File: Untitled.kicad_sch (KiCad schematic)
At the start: 20 parts, among them J1 Battery Connector, J2 Top Screw Terminal, J3 Bottom Screw Terminal, Q1 Q_NMOS_DGS, Q2 Q_NMOS_DGS, Q3 Q_NMOS_DGS, U1 XIAO-ESP32-S3-SMD, U3 LSM6DSO32, U4 MS5611-01BA

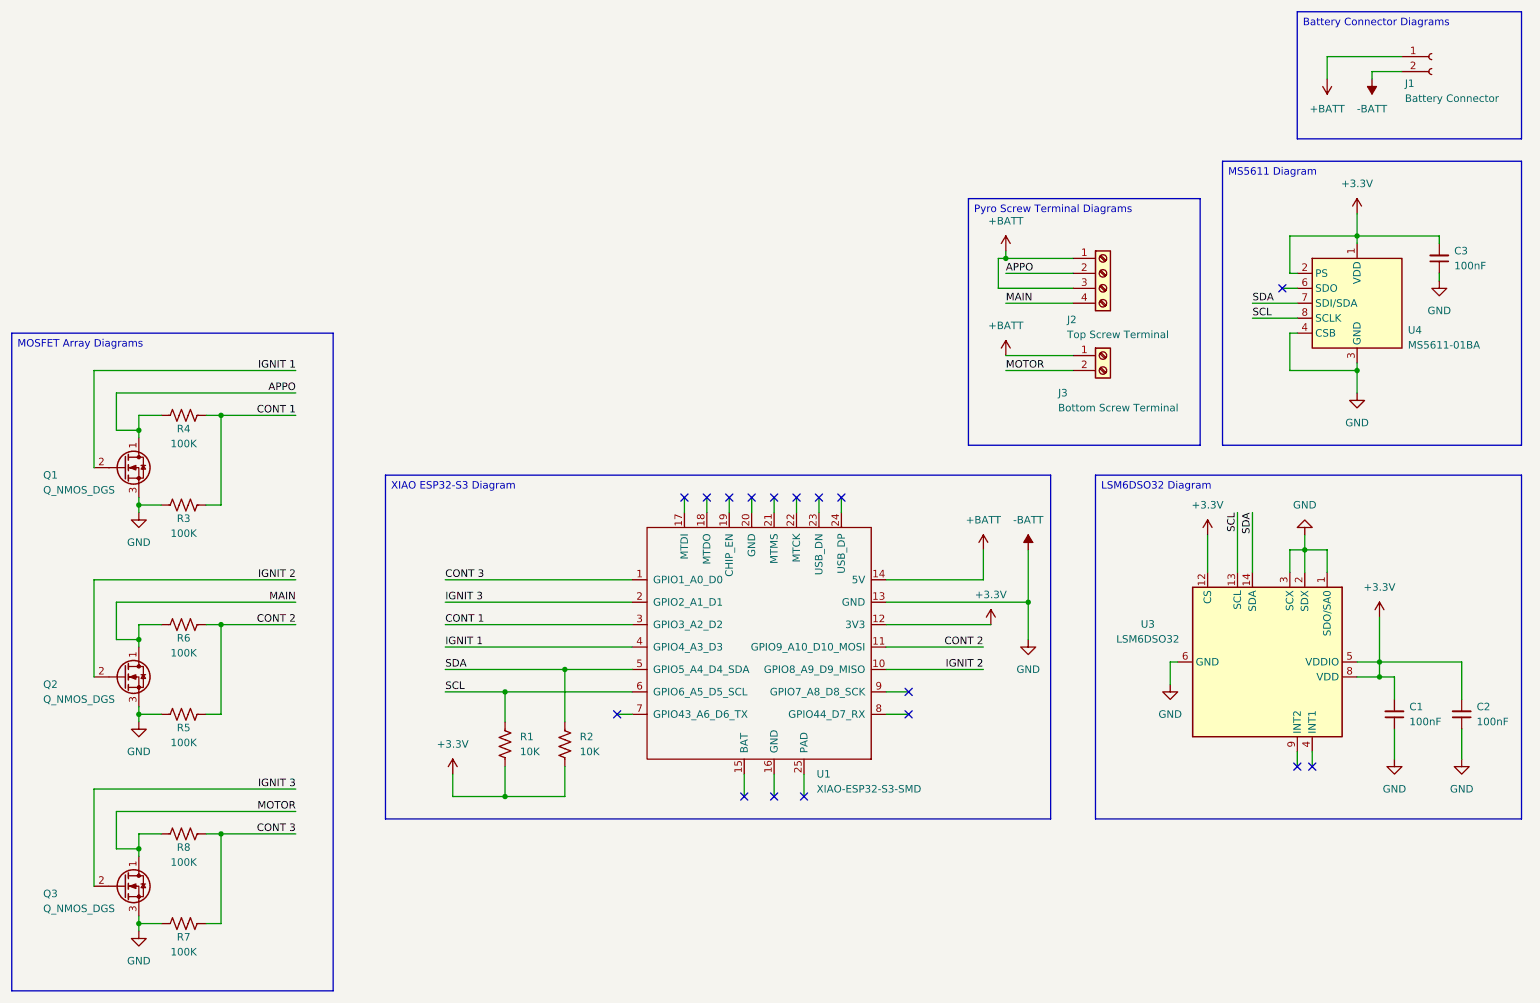
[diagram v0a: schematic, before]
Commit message: Small Changes
Did some small changes to silkscreen formatting.
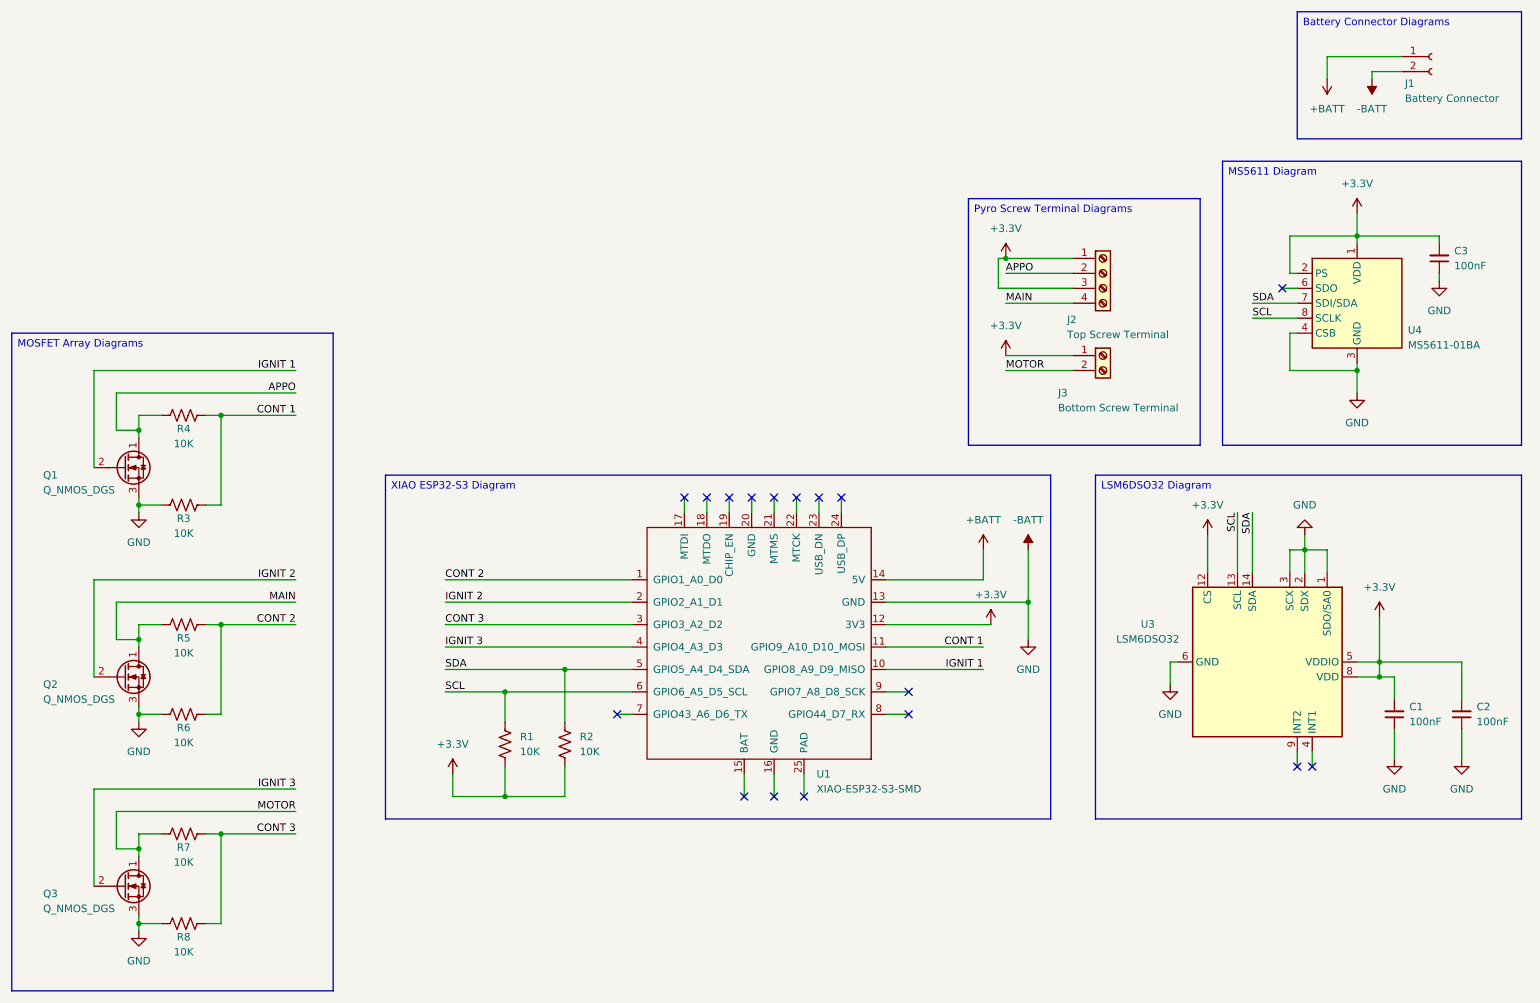
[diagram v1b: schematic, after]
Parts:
- R3, R4: value 100K -> 10K
- R5: renamed from R6; value 100K -> 10K
- R6: renamed from R5; value 100K -> 10K
- R7: renamed from R8; value 100K -> 10K
- R8: renamed from R7; value 100K -> 10K
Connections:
- net +3.3V: now also J2.1 (Pin_1), J2.3 (Pin_3), J3.1 (Pin_1)
- net +BATT: no longer J2.1 (Pin_1), J2.3 (Pin_3), J3.1 (Pin_1)
- net CONT 1: now also U1.11 (GPIO9_A10_D10_MOSI); no longer U1.3 (GPIO3_A2_D2)
- net CONT 2: now also U1.1 (GPIO1_A0_D0); no longer U1.11 (GPIO9_A10_D10_MOSI)
- net CONT 3: now also U1.3 (GPIO3_A2_D2); no longer U1.1 (GPIO1_A0_D0)
- net IGNIT 1: now also U1.10 (GPIO8_A9_D9_MISO); no longer U1.4 (GPIO4_A3_D3)
- net IGNIT 2: now also U1.2 (GPIO2_A1_D1); no longer U1.10 (GPIO8_A9_D9_MISO)
- net IGNIT 3: now also U1.4 (GPIO4_A3_D3); no longer U1.2 (GPIO2_A1_D1)

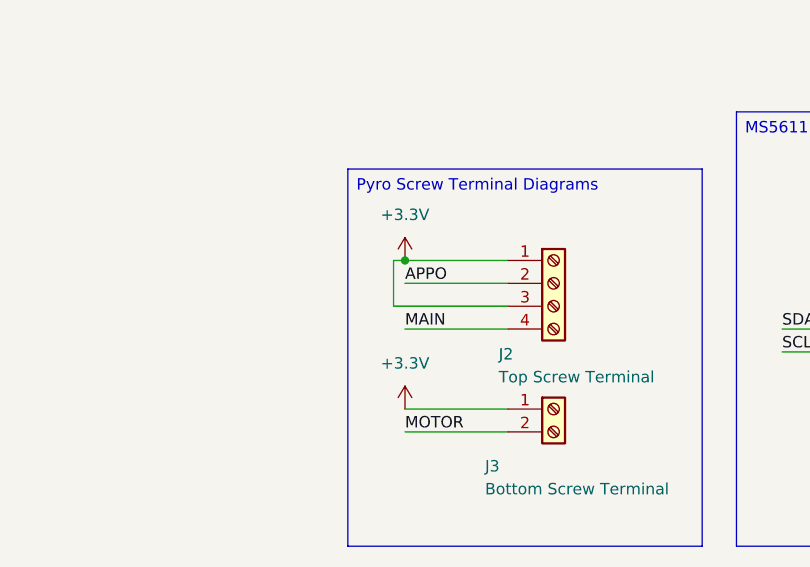
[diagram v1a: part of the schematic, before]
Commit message: Added cutouts, spaced rod holes
Added cutouts to the side of the PCB for wires to pass through on both sides of the ESP32. Changed distance between screw holes to accurately reflect the spacing used for threaded rods on previous avionics designs.
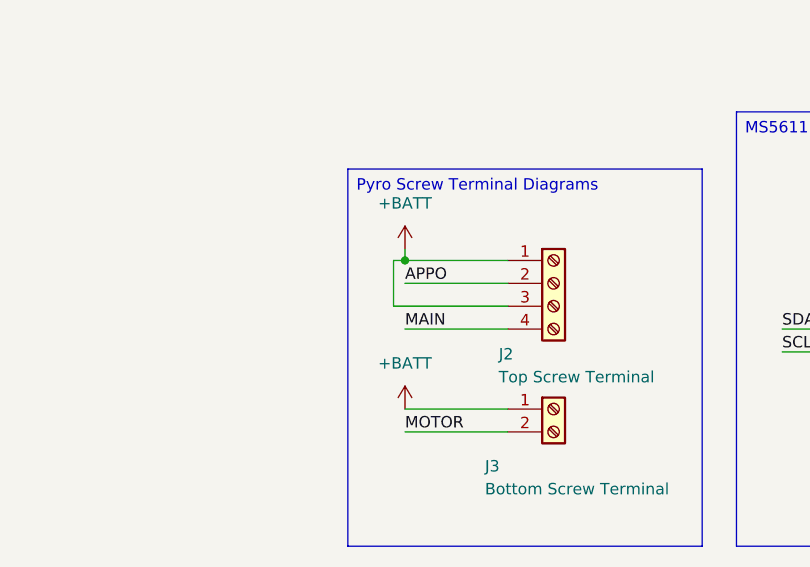
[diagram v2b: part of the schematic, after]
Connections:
- net +3.3V: no longer J2.1 (Pin_1), J2.3 (Pin_3), J3.1 (Pin_1)
- net +BATT: now also J2.1 (Pin_1), J2.3 (Pin_3), J3.1 (Pin_1)

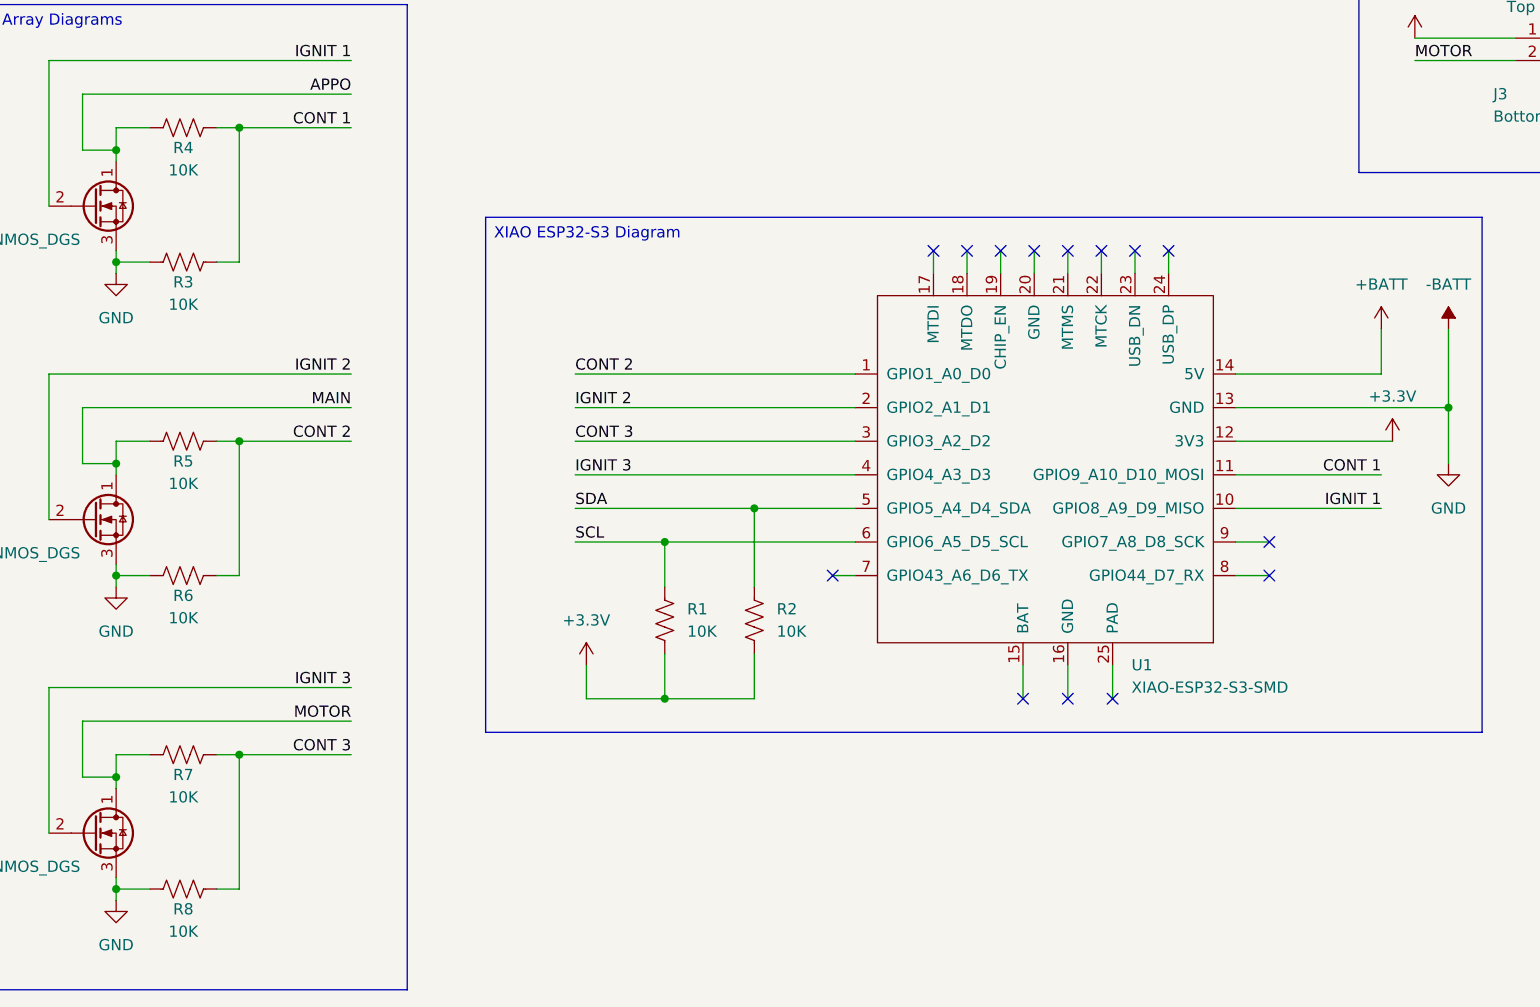
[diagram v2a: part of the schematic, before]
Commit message: Initial Routing
Completed initial manual routing of PCB traces. All nets are fully connected.
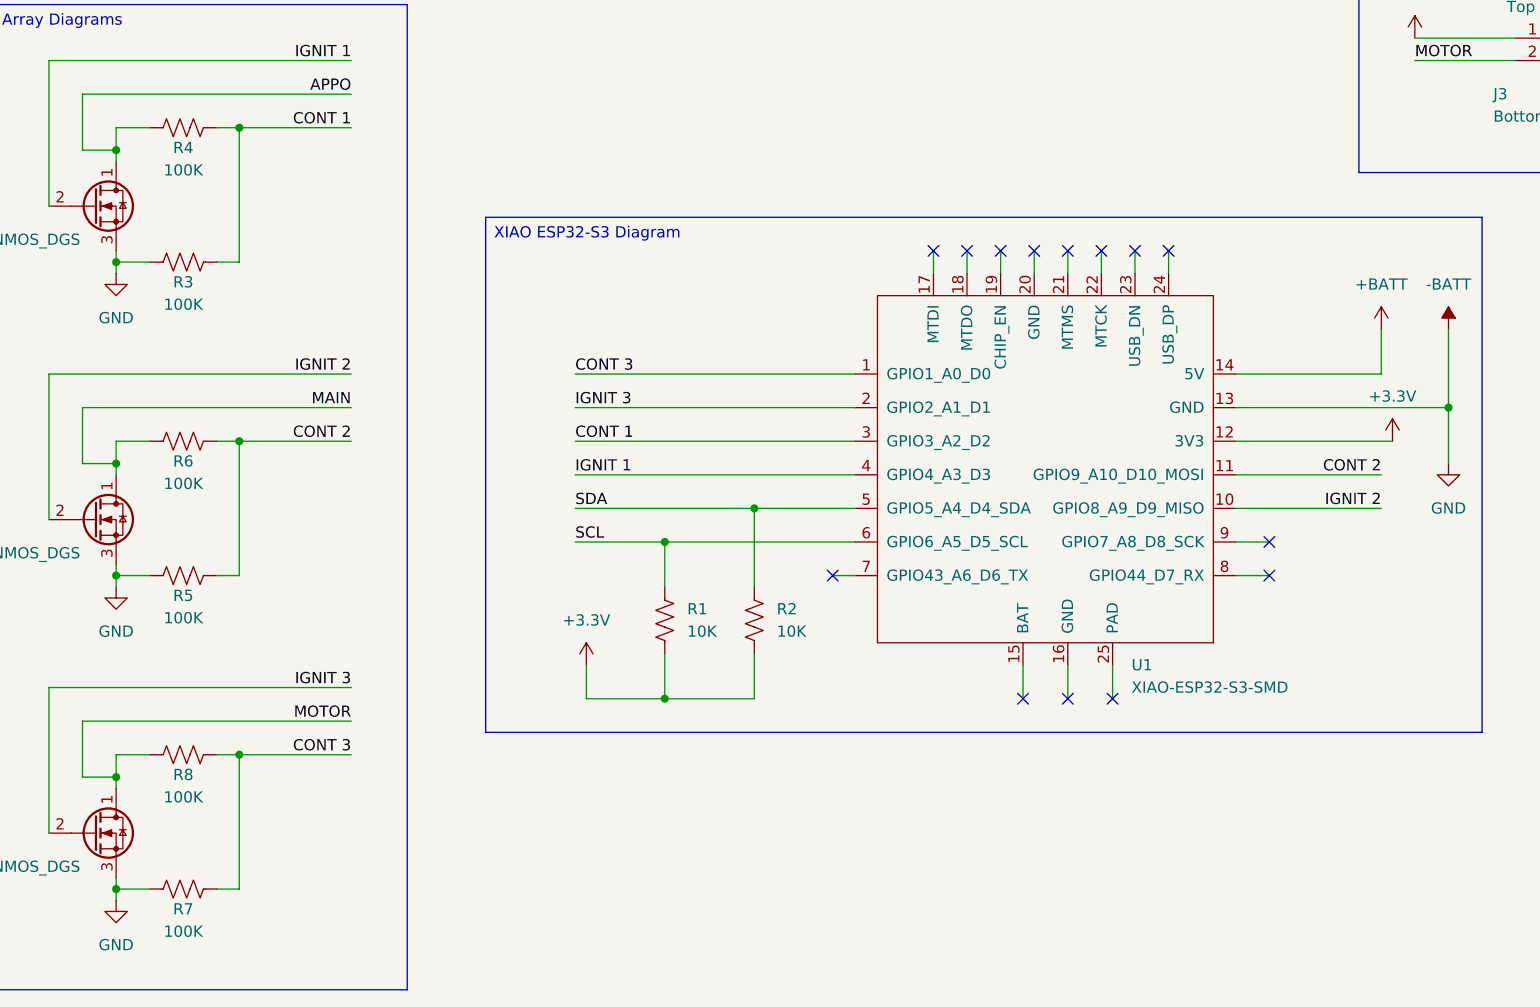
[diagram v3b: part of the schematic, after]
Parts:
- R3, R4: value 10K -> 100K
- R5: renamed from R6; value 10K -> 100K
- R6: renamed from R5; value 10K -> 100K
- R7: renamed from R8; value 10K -> 100K
- R8: renamed from R7; value 10K -> 100K
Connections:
- net CONT 1: now also U1.3 (GPIO3_A2_D2); no longer U1.11 (GPIO9_A10_D10_MOSI)
- net CONT 2: now also U1.11 (GPIO9_A10_D10_MOSI); no longer U1.1 (GPIO1_A0_D0)
- net CONT 3: now also U1.1 (GPIO1_A0_D0); no longer U1.3 (GPIO3_A2_D2)
- net IGNIT 1: now also U1.4 (GPIO4_A3_D3); no longer U1.10 (GPIO8_A9_D9_MISO)
- net IGNIT 2: now also U1.10 (GPIO8_A9_D9_MISO); no longer U1.2 (GPIO2_A1_D1)
- net IGNIT 3: now also U1.2 (GPIO2_A1_D1); no longer U1.4 (GPIO4_A3_D3)
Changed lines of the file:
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@@
 		)
 	)
-	(label "IGNIT 1"
+	(label "IGNIT 2"
 		(at 187.96 137.16 180)
 		(effects
@@
 		)
 	)
-	(label "IGNIT 2"
+	(label "IGNIT 3"
 		(at 96.52 125.73 0)
 		(effects
@@
 		)
 	)
-	(label "CONT 1"
+	(label "CONT 2"
 		(at 187.96 133.35 180)
 		(effects
@@
 		)
 	)
-	(label "IGNIT 3"
+	(label "IGNIT 1"
 		(at 96.52 133.35 0)
 		(effects
@@
 		)
 	)
-	(label "CONT 3"
+	(label "CONT 1"
 		(at 96.52 129.54 0)
 		(effects
@@
 		)
 	)
-	(label "CONT 2"
+	(label "CONT 3"
 		(at 96.52 121.92 0)
 		(effects
@@
 			)
 		)
-		(property "Value" "10K"
+		(property "Value" "100K"
 			(at 52.07 98.806 90)
 			(effects
@@
 		(on_board yes)
 		(dnp no)
-		(property "Reference" "R6"
+		(property "Reference" "R5"
 			(at 52.07 147.066 90)
 			(effects
@@
 			)
 		)
-		(property "Value" "10K"
+		(property "Value" "100K"
 			(at 52.07 149.606 90)
 			(effects
@@
 			(project "Untitled"
 				(path "/de1c2513-dd99-4dc0-9685-67272008b11d"
-					(reference "R6")
+					(reference "R5")
 					(unit 1)
 				)
@@
 			)
 		)
-		(property "Value" "10K"
+		(property "Value" "100K"
 			(at 52.07 114.046 90)
 			(effects
@@
 		(on_board yes)
 		(dnp no)
-		(property "Reference" "R7"
+		(property "Reference" "R8"
 			(at 52.07 167.386 90)
 			(effects
@@
 			)
 		)
-		(property "Value" "10K"
+		(property "Value" "100K"
 			(at 52.07 169.926 90)
 			(effects
@@
 			(project "Untitled"
 				(path "/de1c2513-dd99-4dc0-9685-67272008b11d"
-					(reference "R7")
+					(reference "R8")
 					(unit 1)
 				)
@@
 		(on_board yes)
 		(dnp no)
-		(property "Reference" "R5"
+		(property "Reference" "R6"
 			(at 52.07 131.826 90)
 			(effects
@@
 			)
 		)
-		(property "Value" "10K"
+		(property "Value" "100K"
 			(at 52.07 134.366 90)
 			(effects
@@
 			(project "Untitled"
 				(path "/de1c2513-dd99-4dc0-9685-67272008b11d"
-					(reference "R5")
+					(reference "R6")
 					(unit 1)
 				)
@@
 		(on_board yes)
 		(dnp no)
-		(property "Reference" "R8"
+		(property "Reference" "R7"
 			(at 52.07 182.626 90)
 			(effects
@@
 			)
 		)
-		(property "Value" "10K"
+		(property "Value" "100K"
 			(at 52.07 185.166 90)
 			(effects
@@
 			(project "Untitled"
 				(path "/de1c2513-dd99-4dc0-9685-67272008b11d"
-					(reference "R8")
-					(unit 1)
-				)
+					(reference "R7")
+					(unit 1)
+				)
